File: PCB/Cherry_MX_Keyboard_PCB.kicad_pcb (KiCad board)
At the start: 2 copper layers, 37 parts, among them SW1 MX_1, SW10 MX_7, SW11 MX_11, SW12 MX_15, SW13 MX_4, SW14 MX_8, SW15 MX_12, SW16 MX_16, SW2 MX_5, SW3 MX_9, SW4 MX_13, SW5 MX_2, SW6 MX_6, SW7 MX_10, SW8 MX_14, SW9 MX_3, U1 ARDUINO_PRO_MICRO

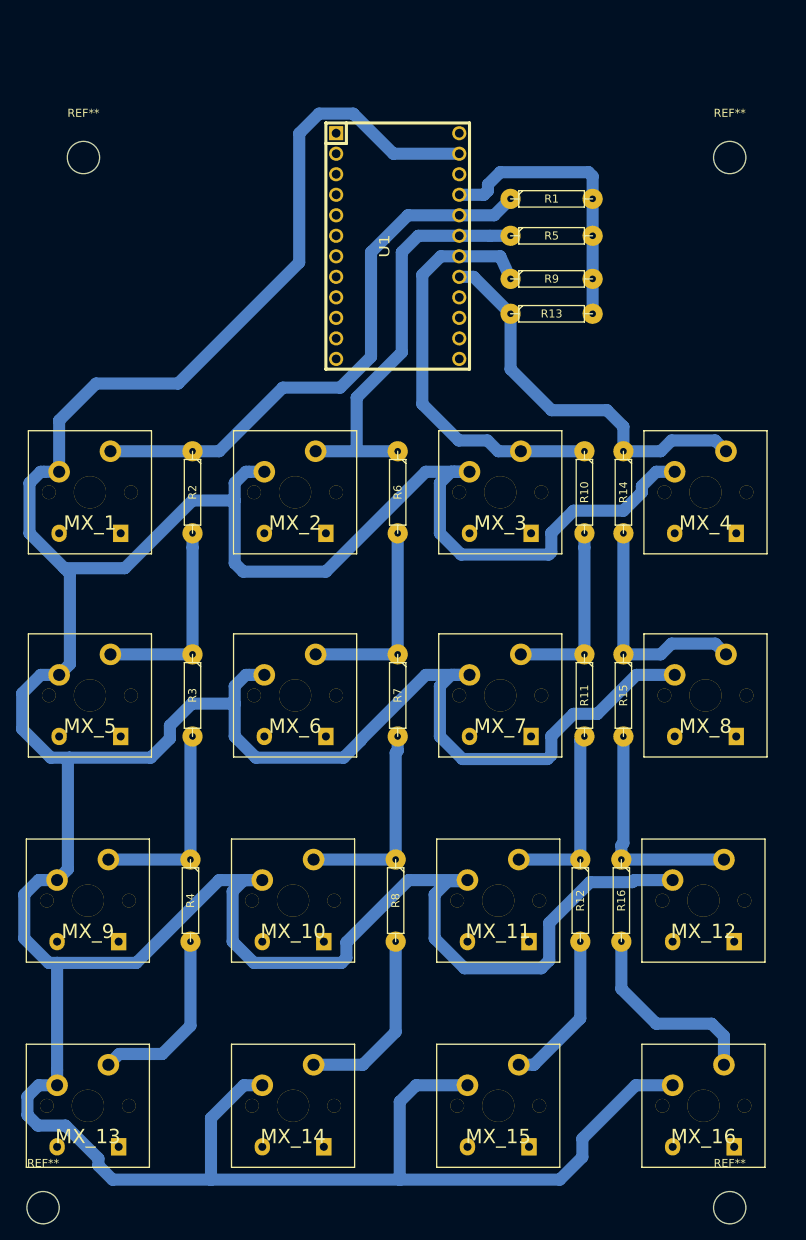
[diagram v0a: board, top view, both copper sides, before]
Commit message: keyboard PCB V 0.2
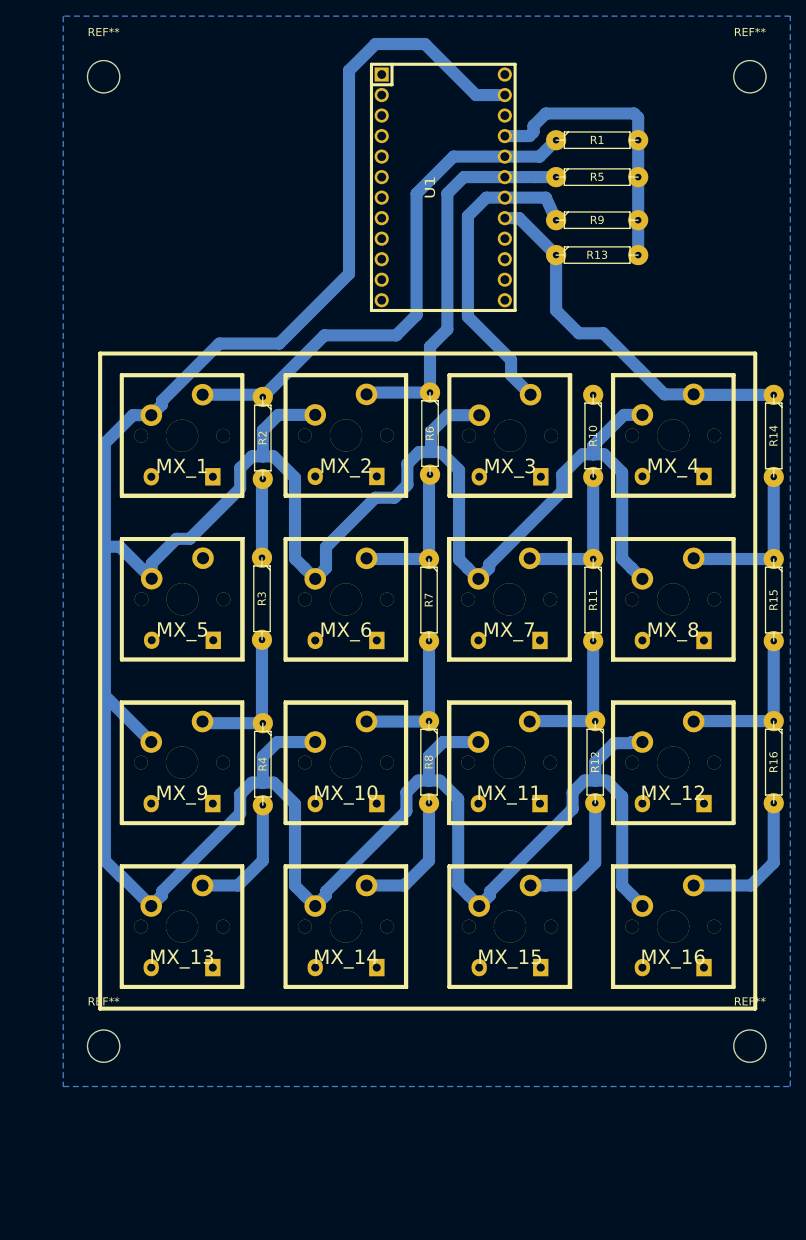
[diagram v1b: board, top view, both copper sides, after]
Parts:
- removed the REF** at (130.0, 180.0)
- removed the REF** at (45.0, 180.0)
- removed the REF** at (50.0, 50.0)
- removed the REF** at (130.0, 50.0)
- added REF**: MountingHole_4mm, Mounting_Holes:MountingHole_4mm, F.Cu at (132.5, 40.0)
- added REF**: MountingHole_4mm, Mounting_Holes:MountingHole_4mm, F.Cu at (52.5, 40.0)
- added REF**: MountingHole_4mm, Mounting_Holes:MountingHole_4mm, F.Cu at (52.5, 160.0)
- added REF**: MountingHole_4mm, Mounting_Holes:MountingHole_4mm, F.Cu at (132.5, 160.0)
- added svg2mod: G***, Cherry_MX_Keyboard:cherryMX, F.Cu at (91.5, 113.5)
- moved R16 25.5 mm to (135.4, 124.8)
- moved SW4 25.1 mm to (62.2, 145.2)
- moved SW8 23.1 mm to (82.5, 145.2)
- moved SW16 22.5 mm to (123.0, 145.2)
- moved SW12 22.2 mm to (102.8, 145.2)
- moved R15 22.0 mm to (135.4, 104.8)
- moved SW3 20.7 mm to (62.2, 124.9)
- moved R14 19.9 mm to (135.4, 84.5)
- moved R4 19.1 mm to (72.2, 125.1)
- moved SW7 18.3 mm to (82.5, 124.9)
- moved R8 17.6 mm to (92.8, 124.8)
- moved SW15 17.5 mm to (123.0, 124.9)
- moved R12 17.2 mm to (113.4, 124.8)
- moved SW11 17.1 mm to (102.7, 124.9)
- moved SW2 16.5 mm to (62.3, 104.7)
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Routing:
- net GND: track 668.1 -> 468.3 mm
- net Net-(R2-Pad2): track 25.1 -> 9.78 mm
- net /ROW_2: track 52.2 -> 39.0 mm
- net Net-(R14-Pad2): track 28.8 -> 20.1 mm
- net Net-(R15-Pad2): track 28.0 -> 19.8 mm
- net Net-(R7-Pad2): track 25.5 -> 17.7 mm
- net Net-(R3-Pad2): track 25.5 -> 17.9 mm
- net Net-(R4-Pad2): track 22.6 -> 15.6 mm
- net Net-(R8-Pad2): track 23.0 -> 16.1 mm
- net Net-(R6-Pad2): track 25.1 -> 18.3 mm
- net Net-(R16-Pad2): track 24.5 -> 18.4 mm
- net Net-(R11-Pad2): track 23.4 -> 18.1 mm
- net Net-(R10-Pad2): track 22.9 -> 18.1 mm
- net /ROW_0: track 70.1 -> 65.8 mm
- net /ROW_1: track 51.4 -> 47.8 mm
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- added copper zone on B.Cu, net GND
